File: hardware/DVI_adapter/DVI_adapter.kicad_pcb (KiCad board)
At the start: 4 copper layers, 34.6 x 28.4 mm, 60 parts, among them J1 DF12NB(3.0)-30DS-0.5V(51), J2 DF12NB(3.0)-30DS-0.5V(51), J3 FPC Cable connector 1x20, U1 TXS0102DQE, U2 HE9009M6R, U3 TFP410

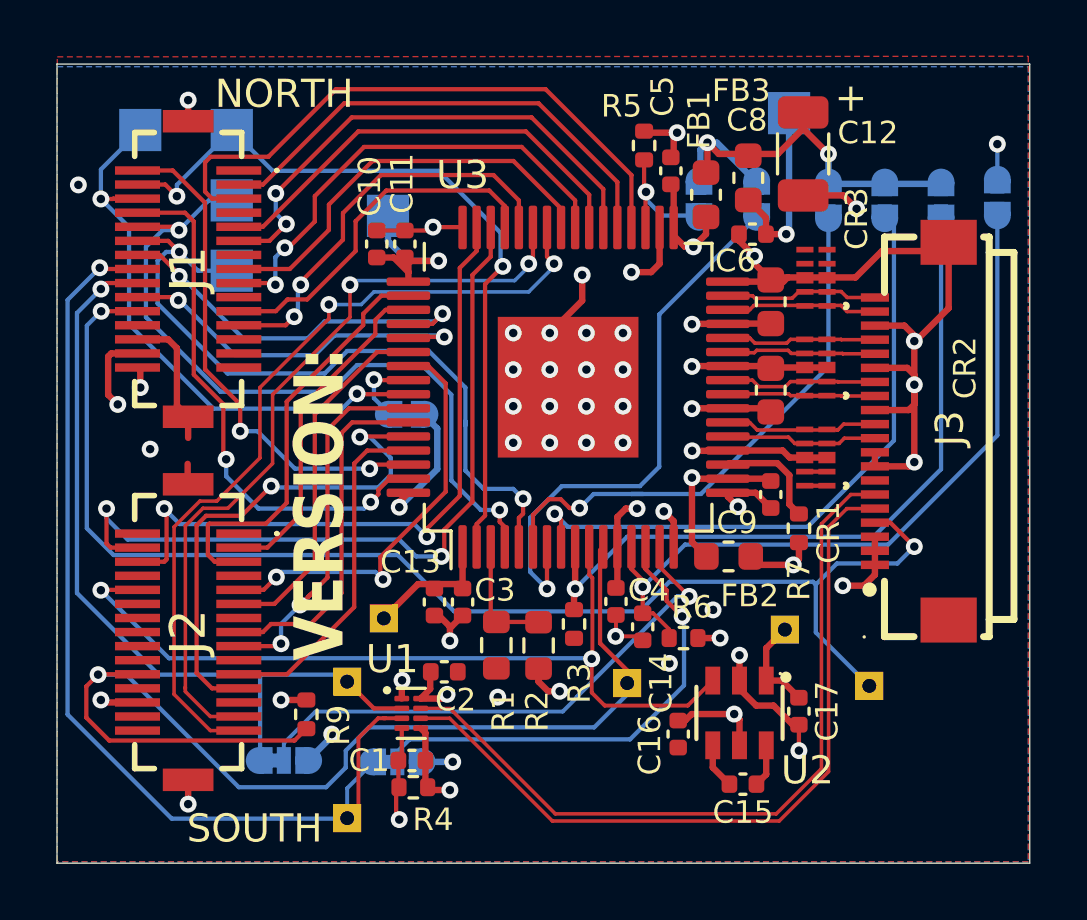
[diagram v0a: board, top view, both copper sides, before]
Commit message: fixes for producion and notes
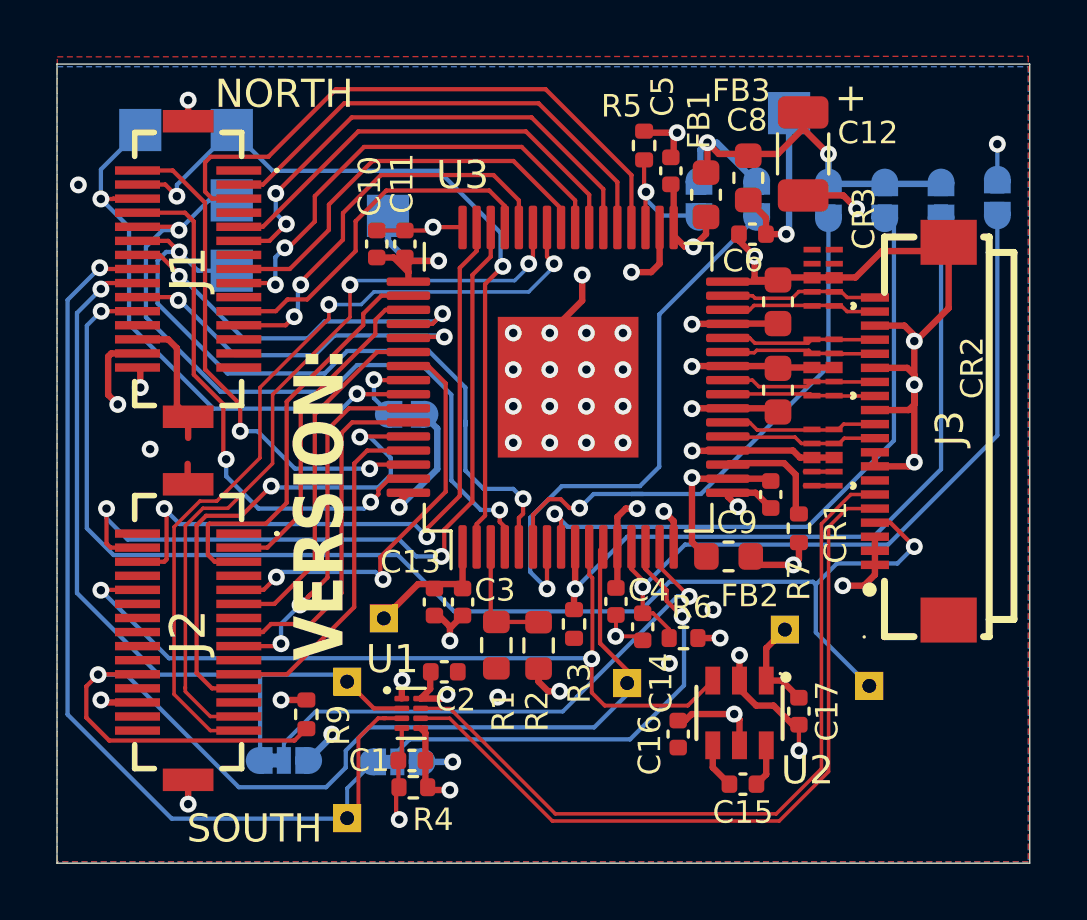
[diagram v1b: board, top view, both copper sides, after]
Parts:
- moved C6 0.26 mm to (129.4, 121.4)
- moved C7 0.26 mm to (129.4, 124.5)
- moved CR1 0.26 mm to (131.0, 126.9)
- moved CR2 0.26 mm to (131.0, 123.7)
- moved CR3 0.26 mm to (131.0, 120.5)
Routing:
- net /TX0-: track 6.05 -> 5.26 mm
- net TVDD: track 24.8 -> 25.4 mm
